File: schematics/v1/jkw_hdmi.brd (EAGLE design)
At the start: 30 parts, among them J1 2X20-CHIP-HEADERS, J2 T_MOLEX_45171, U1 DS2431P

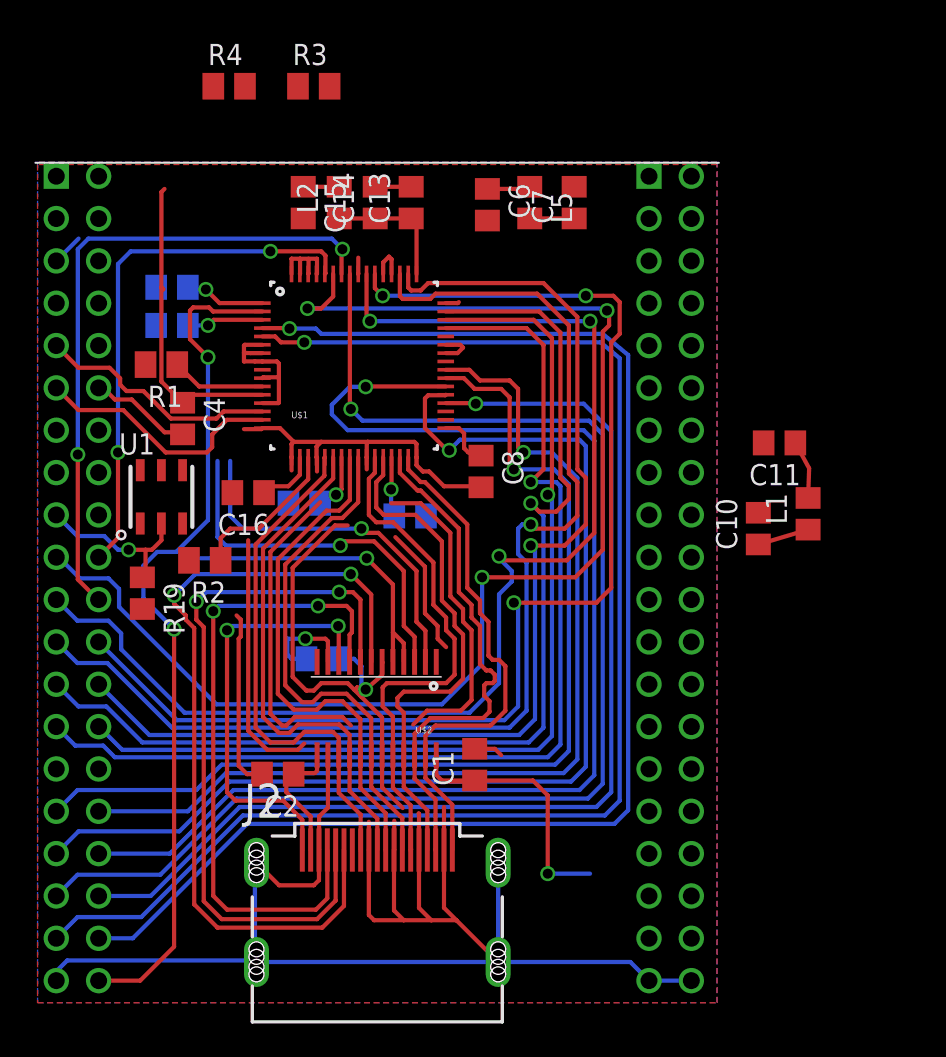
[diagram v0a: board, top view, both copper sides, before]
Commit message: layout 1
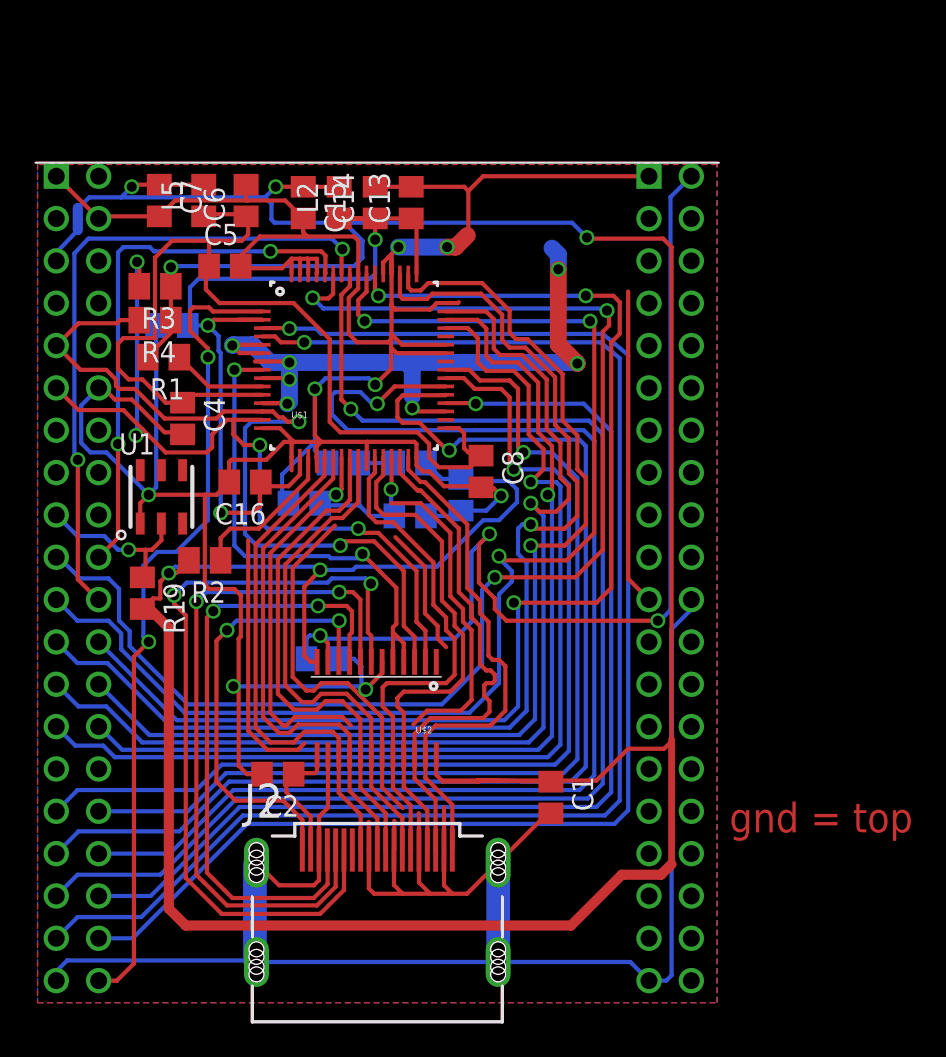
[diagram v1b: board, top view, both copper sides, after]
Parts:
- moved C10 25.2 mm to (29.9, 36.2), flipped to the bottom, turned to 0 degrees
- moved C7 24.9 mm to (18.9, 51.9), turned to 270 degrees
- moved L1 24.1 mm to (33.9, 36.2), flipped to the bottom, turned to 180 degrees
- moved L5 19.6 mm to (21.5, 51.9), turned to 90 degrees
- moved C11 19.4 mm to (37.0, 34.3), flipped to the bottom, turned to 270 degrees
- moved R3 15.3 mm to (18.6, 46.8), turned to 180 degrees
- moved R4 14.7 mm to (18.6, 44.8), turned to 180 degrees
- moved C6 14.5 mm to (24.1, 51.9), turned to 90 degrees
- moved C1 4.98 mm to (42.4, 16.1), turned to 270 degrees
- moved C5 3.42 mm to (22.8, 48.0), flipped to the top
- moved C16 0.66 mm to (24.0, 35.1)
- moved R1 0.46 mm to (19.1, 42.5)
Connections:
- net VCC-5V: now also J1.VCC5V@0; no longer J1.VCC5V@1
- net VCC_5V_DCC: now also J1.VCC5V@1; no longer J1.VCC5V@0
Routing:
- net VCC: track 38.1 -> 270.2 mm, vias 1 -> 13
- net GND: track 210.0 -> 365.9 mm, vias 1 -> 8
- net VCC_5V_DCC: track 5.94 -> 62.0 mm, vias 1 -> 3
- net N$10: track 16.0 -> 52.4 mm, vias 1 -> 3
- net N$4: track 29.4 -> 59.4 mm, vias 1 -> 0
- net N$14: track 0.00 -> 19.5 mm
- net TWI1_SCK: track 36.7 -> 51.4 mm, vias 1 -> 4
- net TWI1_SDA: track 37.1 -> 48.8 mm, vias 1 -> 2
- net HOTPLUG_DET: track 18.9 -> 29.8 mm, vias 1 -> 2
- net N$13: track 0.00 -> 7.87 mm
- net N$8: track 10.3 -> 16.6 mm
- net LCD-D22: track 67.0 -> 69.9 mm
- net LCD-DE: track 51.5 -> 49.5 mm
- net N$6: track 44.0 -> 42.2 mm
- net LCD-D11: track 66.9 -> 65.2 mm
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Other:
- board text added: "gnd = top"

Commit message: improved silk
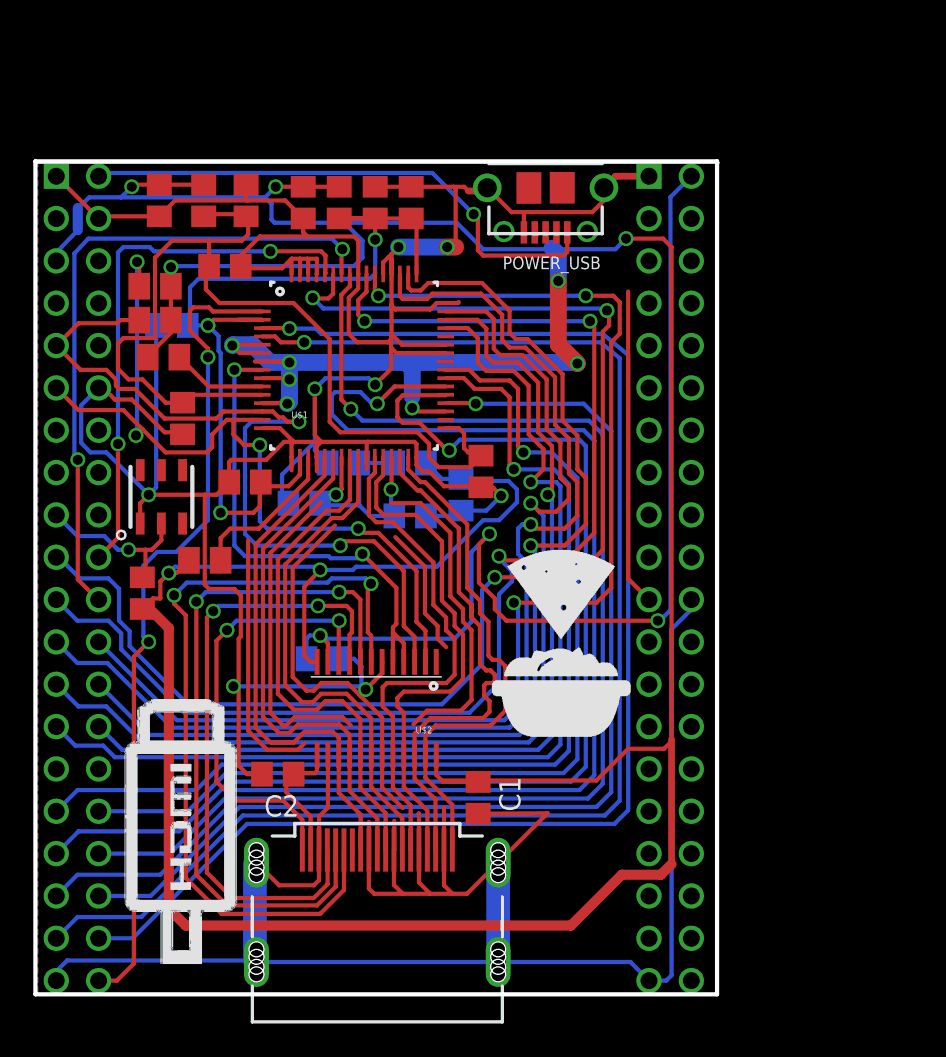
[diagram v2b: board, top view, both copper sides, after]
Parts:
- added POWER_USB: USBUSB-MICROB-SMT-DIP, Spark:USB-MICROB-SMT-DIP
- added U$3: LOGO_10X10_SILK, logo:LOGO_10X10_SILK
- added U$4: LOGO_25X25_SILK, logo:LOGO_25X25_SILK
- moved C1 4.37 mm to (38.0, 16.1)
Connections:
- removed net N$1: J1.CHG-IN
- new net VOUT: J1.CHG-IN, POWER_USB.VBUS
- net GND: now also POWER_USB.GND, POWER_USB.MT1, POWER_USB.MT2
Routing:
- net VOUT: track 0.00 -> 32.6 mm, vias 0 -> 1
- net GND: track 365.9 -> 372.8 mm
- net VCC: track 270.2 -> 266.5 mm
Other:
- board outline added: 40.9 x 50 mm
- board text removed: "gnd = top"

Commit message: improved silk
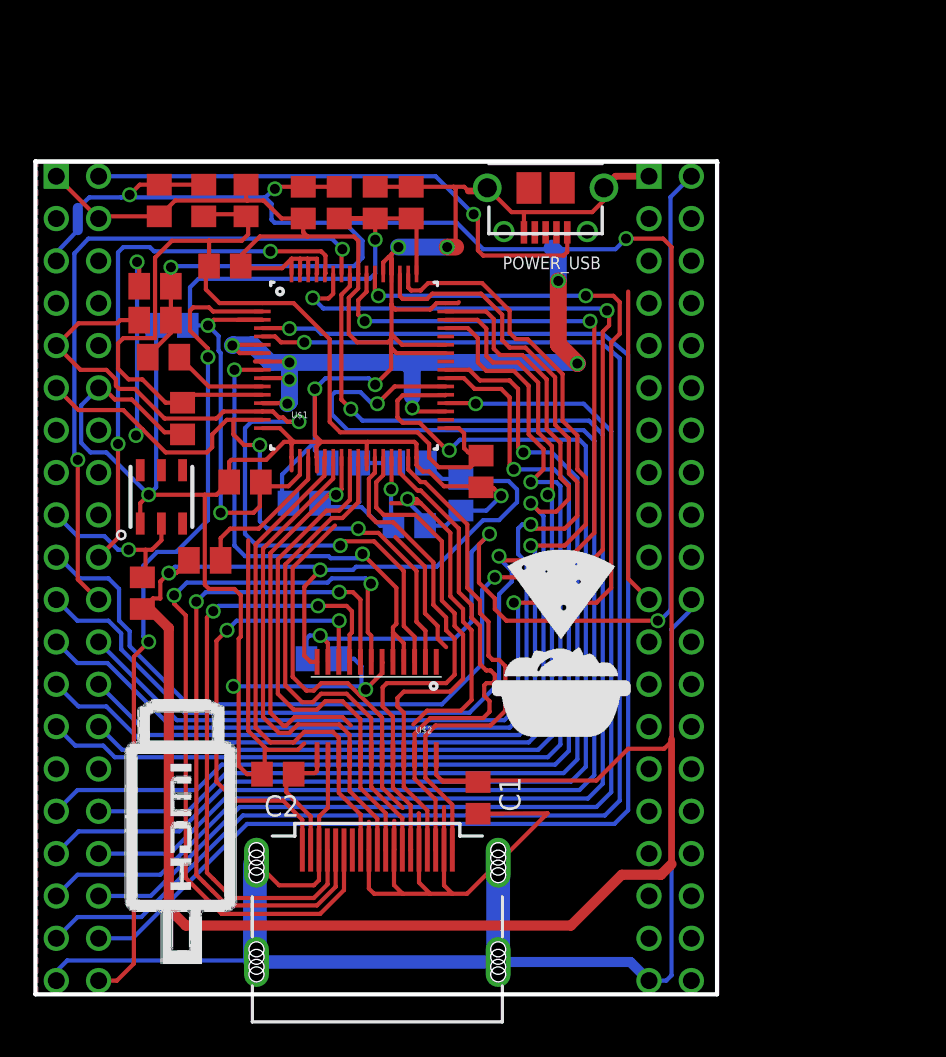
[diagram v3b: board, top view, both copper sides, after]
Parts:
- moved C12 0.59 mm to (33.9, 32.4)
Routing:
- net GND: track 372.8 -> 412.7 mm, vias 8 -> 9
- net N$8: track 16.6 -> 39.0 mm
- net N$14: track 19.5 -> 0.00 mm
- net N$11: track 18.9 -> 0.00 mm
- net N$12: track 15.4 -> 0.00 mm
